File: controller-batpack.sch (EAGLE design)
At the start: 7 parts

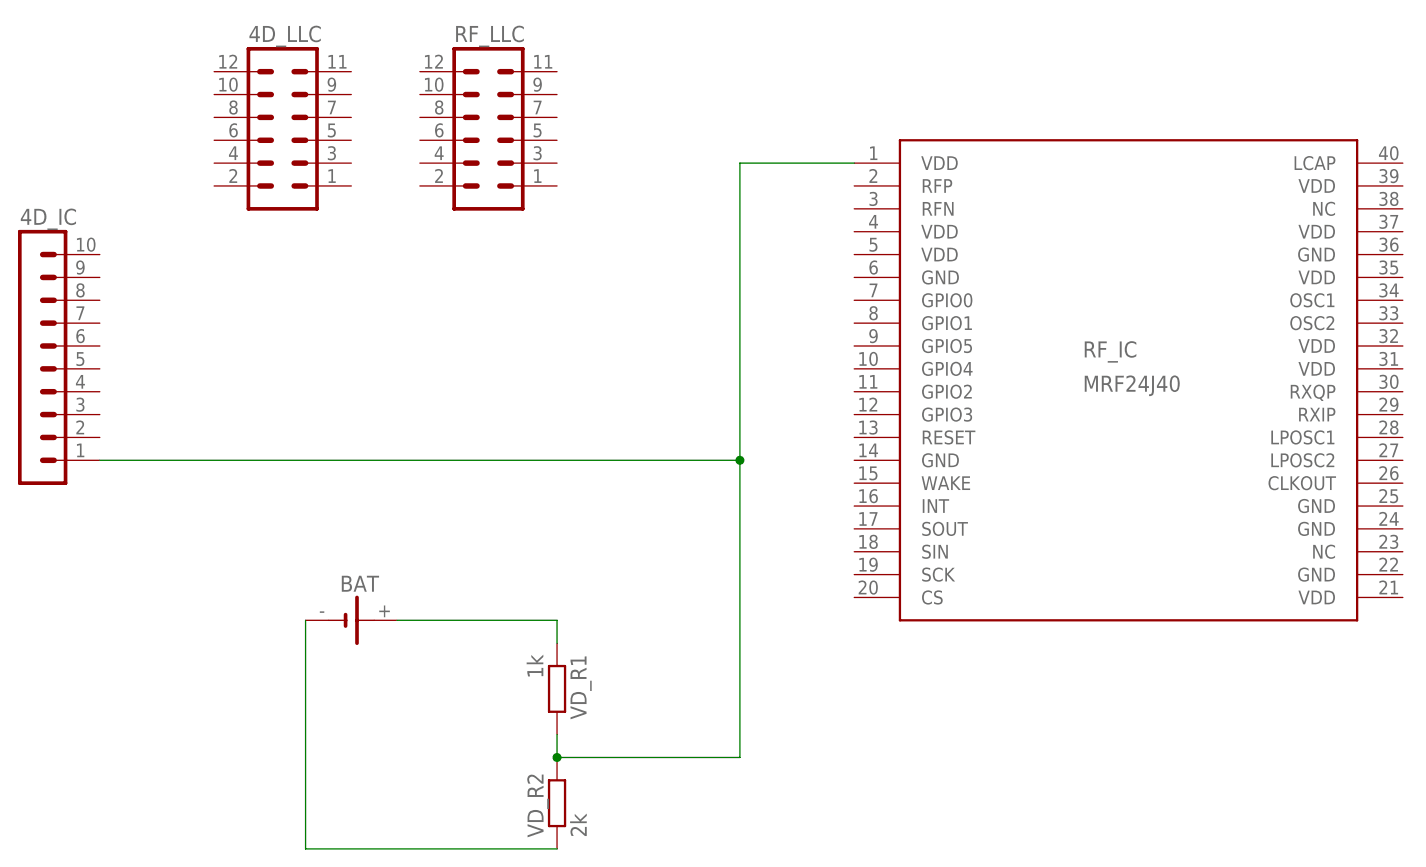
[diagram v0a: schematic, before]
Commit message: updated board with display and battery
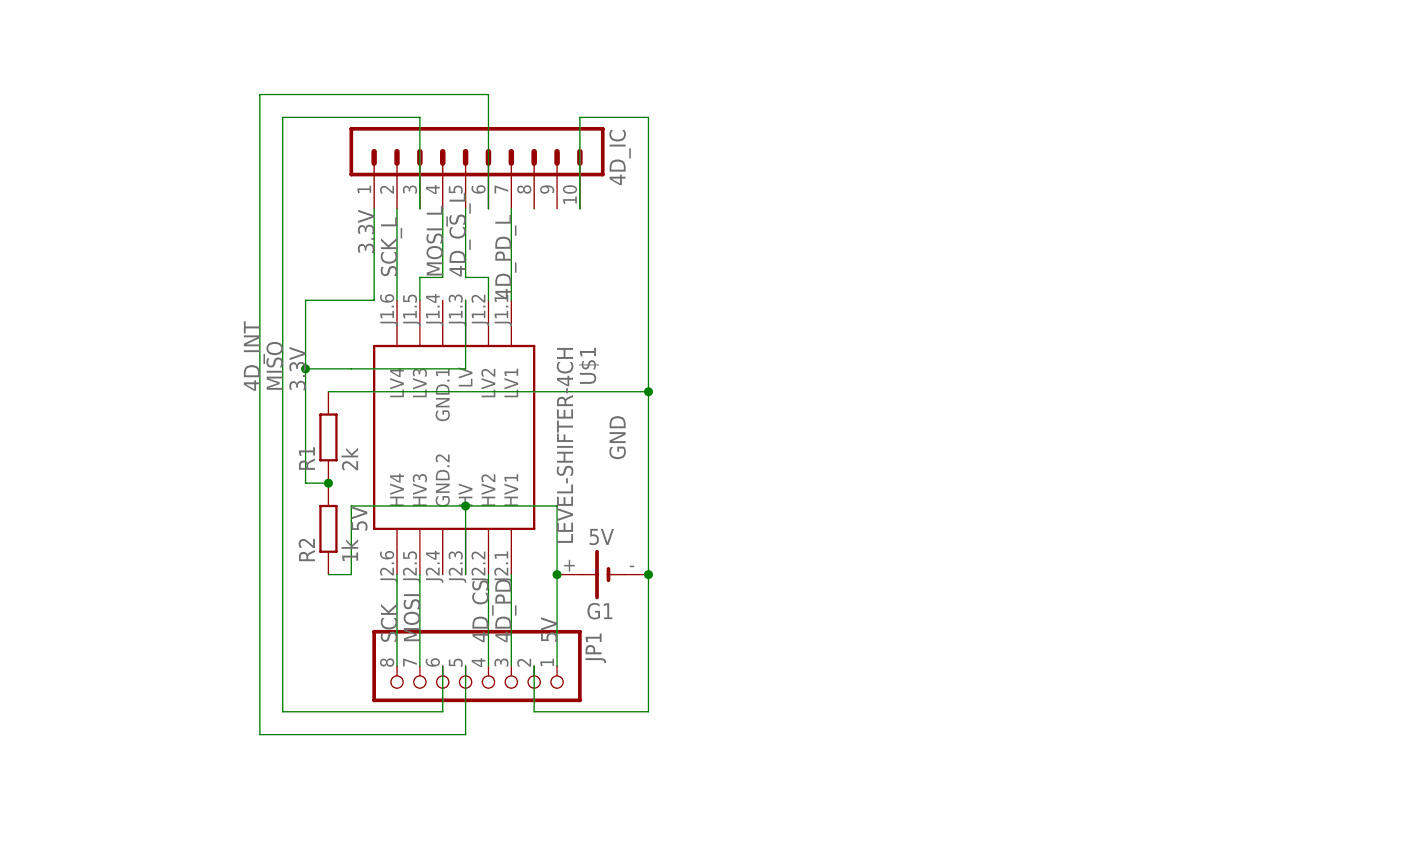
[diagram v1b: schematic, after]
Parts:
- removed 4D_LLC, RF_LLC: (no value), con-lstb:MA06-2
- removed BAT: SL-160AA/PR, battery:SL-160AA/PR
- removed RF_IC: MRF24J40, microchip:MRF24J40
- removed VD_R1: 1k, resistor:R-EU_0204/5
- removed VD_R2: 2k, resistor:R-EU_0204/5
- added G1: 5V, battery:SL-160AA/PR
- added JP1: (no value), pinhead:PINHD-1X8
- added R1: 2k, rcl:R-EU_0204/5
- added R2: 1k, rcl:R-EU_0204/5
- added U$1: LEVEL-SHIFTER-4CH, diy-modules:LEVEL-SHIFTER-4CH
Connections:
- removed net N$1: BAT.-, VD_R2.1
- removed net N$2: BAT.+, VD_R1.1
- removed net N$3: 4D_IC.1, RF_IC.VDD, VD_R1.2, VD_R2.2
- new net 3.3V: 4D_IC.1, R1.1, R2.2
- new net 4D_CS: JP1.4, U$1.HV2
- new net 4D_CS_L: 4D_IC.5, U$1.LV2
- new net 4D_INT: 4D_IC.6, JP1.5
- new net 4D_PD: JP1.3, U$1.HV1
- new net 4D_PD_L: 4D_IC.7, U$1.LV1
- new net 5V: G1.+, JP1.1, R2.1, U$1.HV
- new net GND: 4D_IC.10, G1.-, JP1.2, R1.2
- new net MISO: 4D_IC.3, JP1.6
- new net MOSI: JP1.7, U$1.HV3
- new net MOSI_L: 4D_IC.4, U$1.LV3
- new net N$10: U$1.LV
- new net SCK: JP1.8, U$1.HV4
- new net SCK_L: 4D_IC.2, U$1.LV4
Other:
- moved on the sheet: 4D_IC
